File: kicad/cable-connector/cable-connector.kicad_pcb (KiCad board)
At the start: 2 copper layers, 90 x 65 mm, 11 parts, among them J1 Conn_01x04_Pin, J10 Conn_01x04_Pin, J11 Conn_01x04_Pin, J2 Conn_01x04_Pin, J3 Conn_01x04_Pin, J4 Conn_01x04_Pin, J5 Conn_01x04_Pin, J6 Conn_01x04_Pin, J7 Conn_01x04_Pin, J8 Conn_01x04_Pin, J9 Conn_01x04_Pin

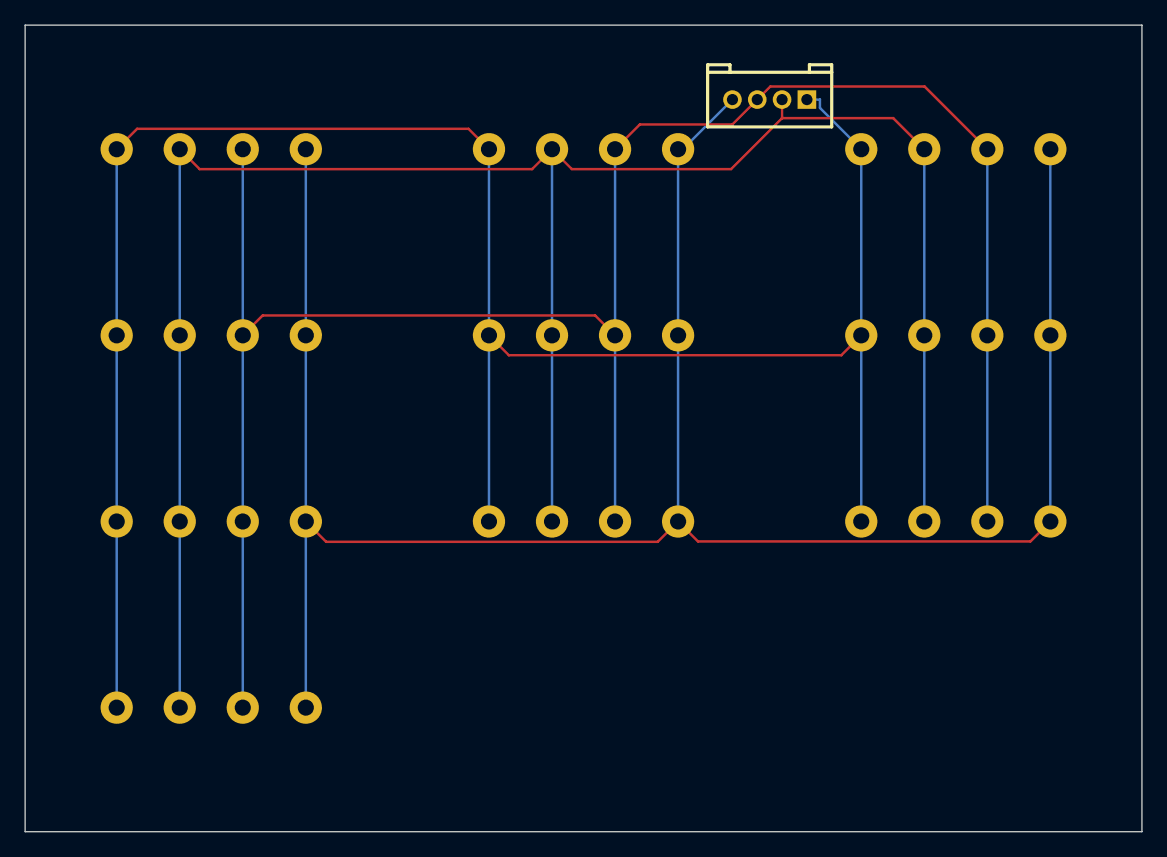
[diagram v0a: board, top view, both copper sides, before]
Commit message: The Academy
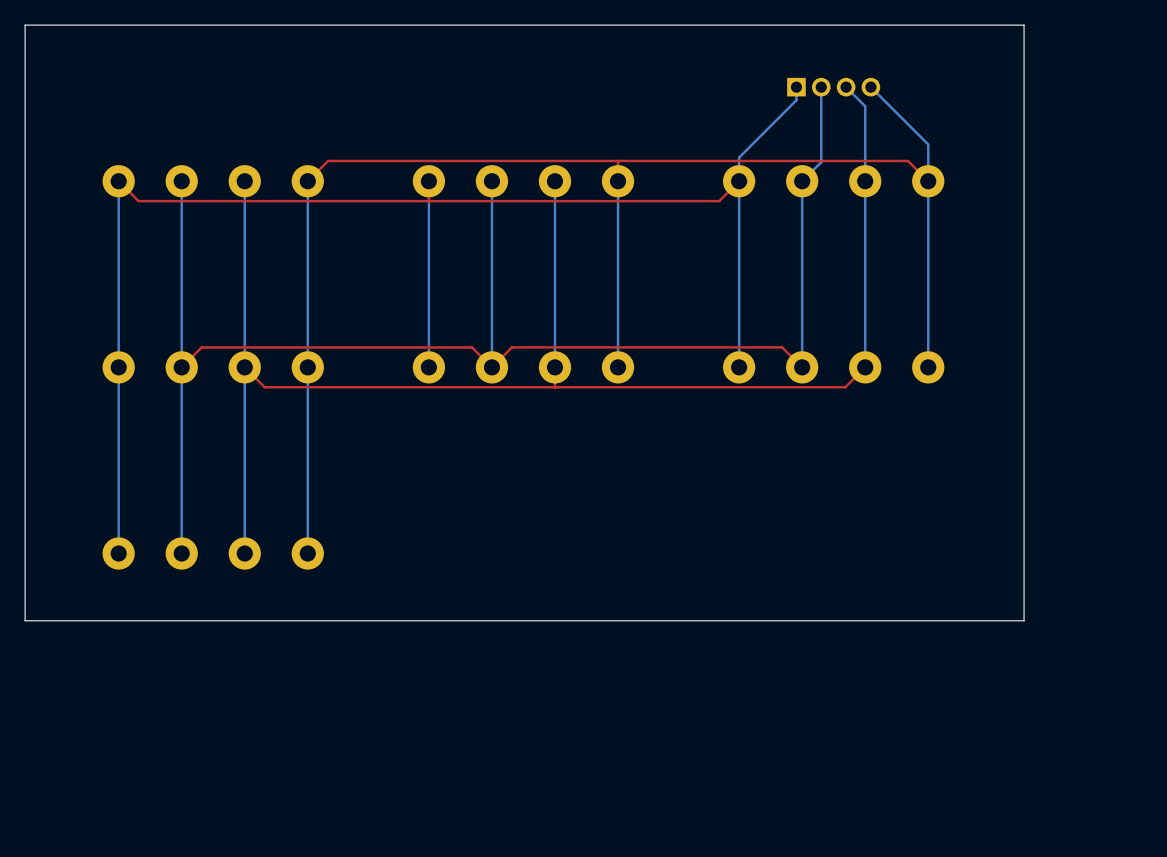
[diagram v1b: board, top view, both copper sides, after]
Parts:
- removed J10, J9: Conn_01x04_Pin, footprints:SDI_Connector
- removed J11: Conn_01x04_Pin, footprints:GROVE-HW4-2.0
- J8: footprint footprints:SDI_Connector -> footprints:GROVE-HW4-2.0; moved to B.Cu
- moved J3 57.2 mm to (140.2, 77.6)
- moved J7 30.0 mm to (90.2, 107.6)
- moved J2 28.1 mm to (115.2, 77.6)
- moved J4 27.4 mm to (90.2, 92.6)
- moved J6 20.3 mm to (140.2, 92.6)
- moved J5 18.2 mm to (115.2, 92.6)
- moved J8 11.0 mm to (140.2, 70.0)
- moved J1 2.58 mm to (90.2, 77.6)
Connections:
- net /BLACK renamed LINE
- net /BLUE renamed VBUS
- net /BROWN renamed GND
- net /WHITE renamed +12V
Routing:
- net VBUS: track 174.1 -> 122.4 mm
- net LINE: track 173.7 -> 122.5 mm
- net +12V: track 171.2 -> 120.9 mm
- net GND: track 170.5 -> 121.1 mm
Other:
- board size 90 x 65 mm -> 80.5 x 48 mm
